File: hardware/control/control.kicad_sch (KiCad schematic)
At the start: 58 parts, among them J1 Conn_01x05_Male, J2 CANPWR, J3 CANGND, J4 RJ45, J5 RJ45, J6 Conn_02x03_Odd_Even, J7 DCDC-PWM, J8 DCDC-MEASURES, Q1 BSS123, SW1 next, SW2 select, U1 2.048V, U2 AP63200WU, U3 PIC18F27Q84, U4 TLE9250VSJXUMA1, Y1 10Mhz

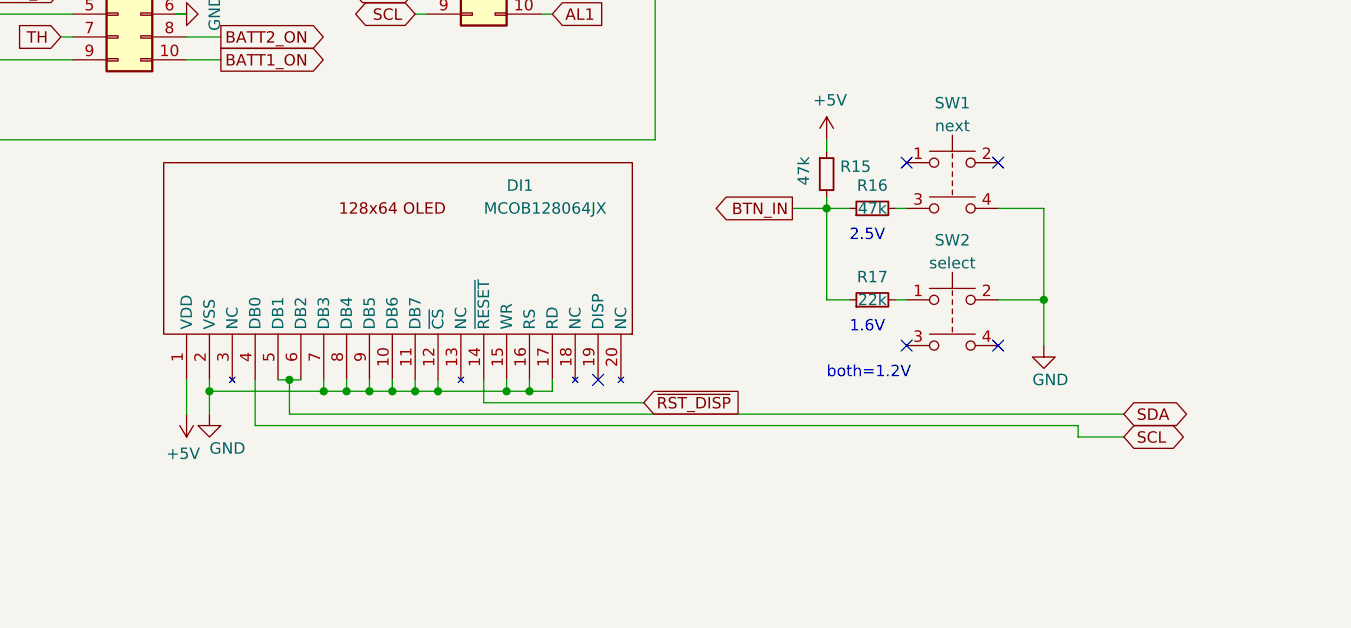
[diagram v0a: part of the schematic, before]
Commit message: WIP on diaplay PCB.
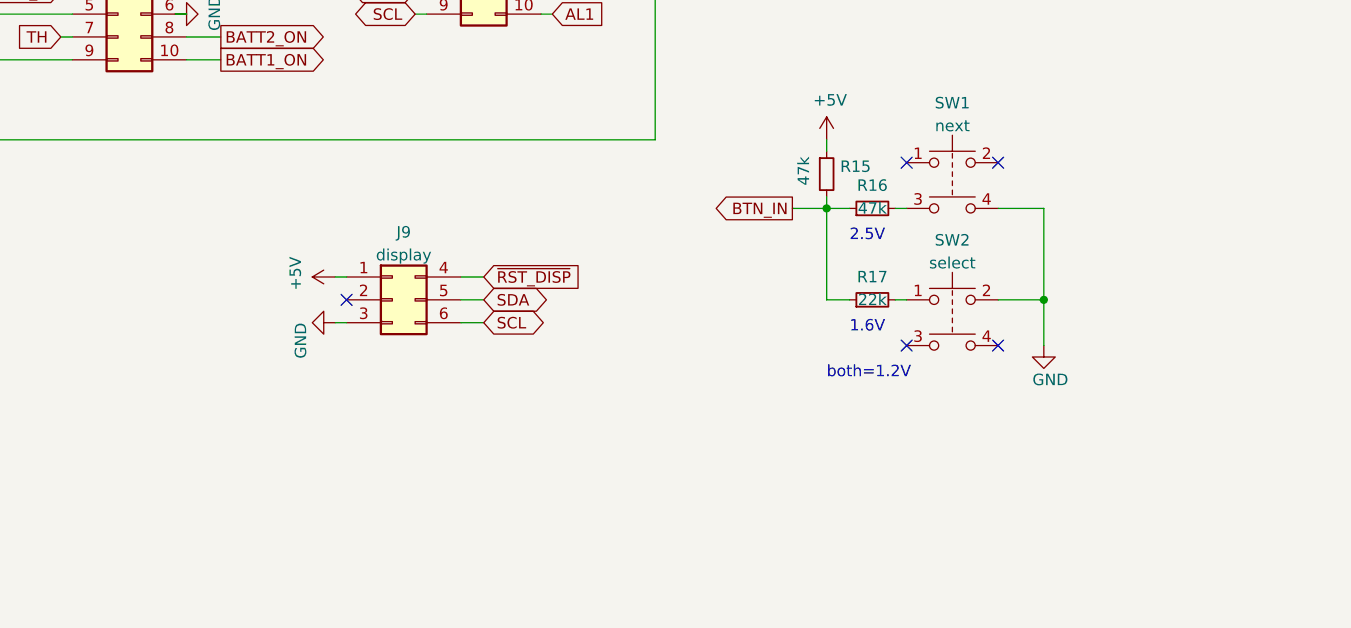
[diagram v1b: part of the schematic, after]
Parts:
- removed DI1: MCOB128064JX, LCDdisplays.mod:MCOB128064JX, symbol LCDdisplays:MCOB128064JX
- added J9: display, Connector_Harwin:Harwin_M20-7810345_2x03_P2.54mm_Vertical, symbol Connector_Generic:Conn_02x03_Top_Bottom
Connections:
- net +5V: now also J9.1 (Pin_1)
- net GND: now also J9.3 (Pin_3)
- net SCL: now also J9.6 (Pin_6)
- net SDA: now also J9.5 (Pin_5)
- net ~{RST_DISP}: now also J9.4 (Pin_4)
